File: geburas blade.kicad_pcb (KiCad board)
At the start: 2 copper layers, 71.8 x 71.8 mm, 17 parts, among them M1 Motor_DC, Q1 2N3904, SW2 SW_Push, U2 ICM7555xP

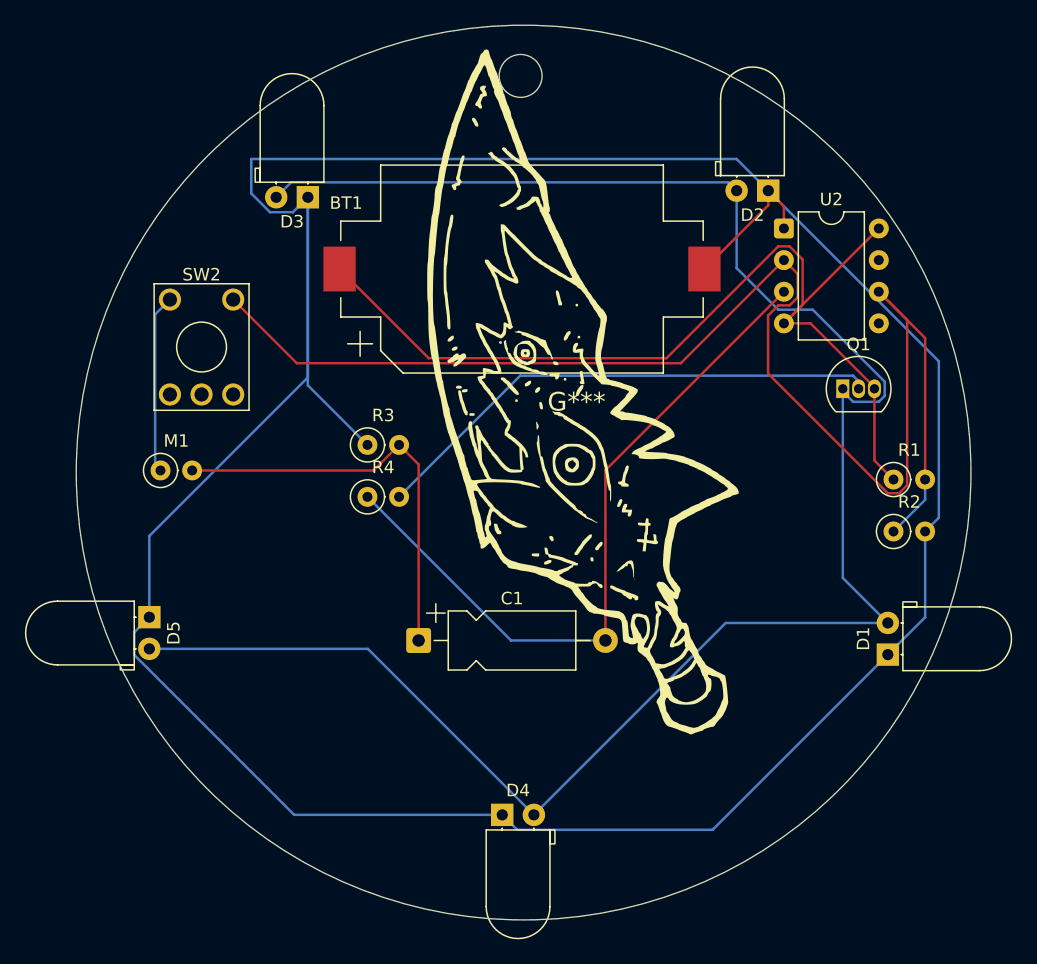
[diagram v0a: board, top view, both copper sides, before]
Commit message: Add files via upload
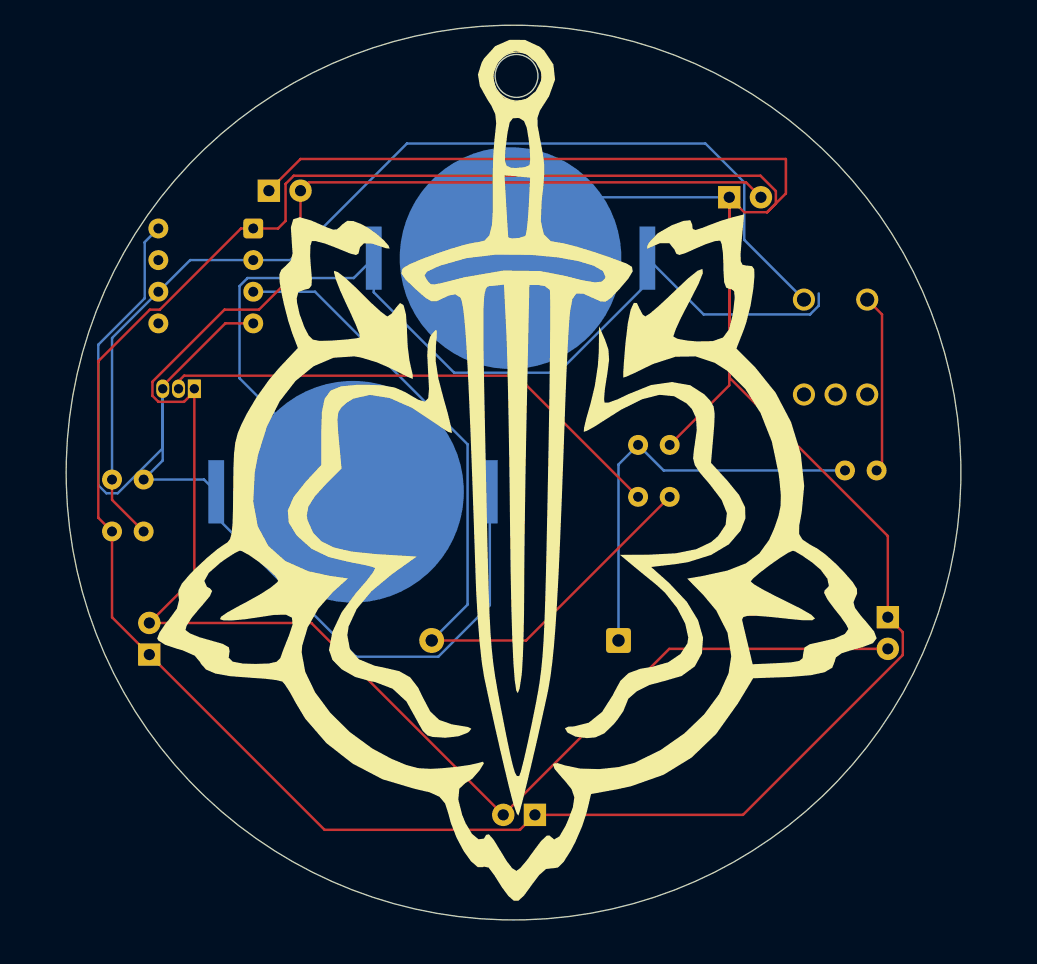
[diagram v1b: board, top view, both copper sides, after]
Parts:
- added BT2: Battery_Cell, Battery:BatteryHolder_Keystone_3034_1x20mm, B.Cu at (128.5, 76.5)
- BT1: footprint Battery:BatteryHolder_Keystone_1060_1x2032 -> Battery:BatteryHolder_Keystone_3034_1x20mm; moved to B.Cu
- C1, D1, D2, D3, D4, D5, G***, M1, Q1, R1, R2, R3, R4, SW2, U2: moved to B.Cu
- G***: moved to F.Cu
- moved R1 60.2 mm to (111.7, 75.5), turned to 180 degrees
- moved R2 60.2 mm to (111.7, 79.7), turned to 180 degrees
- moved D1 59.3 mm to (112.2, 89.5)
- moved D5 59.3 mm to (171.5, 86.5)
- moved M1 57.5 mm to (170.6, 74.8), turned to 180 degrees
- moved SW2 56.0 mm to (169.8, 61.0), turned to 180 degrees
- moved Q1 52.1 mm to (115.8, 68.2), turned to 180 degrees
- moved U2 42.6 mm to (120.5, 55.3), turned to 180 degrees
- moved D2 40.1 mm to (121.8, 52.3), turned to 0 degrees
- moved D3 33.8 mm to (158.8, 52.8), turned to 0 degrees
- moved R3 24.3 mm to (154.0, 72.7), turned to 180 degrees
- moved R4 24.3 mm to (154.0, 76.9), turned to 180 degrees
- moved C1 16.1 mm to (149.9, 88.4), turned to 180 degrees
- moved G*** 9.31 mm to (137.2, 69.3), turned to 180 degrees
- moved D4 2.62 mm to (143.1, 102.4), turned to 180 degrees
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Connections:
- Q1 pad 3: Net-(BT1-+) -> Net-(BT2-+)
- R1 pad 1: Net-(BT1-+) -> Net-(BT2-+)
- U2 pad 4: Net-(BT1-+) -> Net-(BT2-+)
- U2 pad 8: Net-(BT1-+) -> Net-(BT2-+)
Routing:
- net Net-(BT2-+): track 0.00 -> 97.6 mm
- net Net-(BT1--): track 244.1 -> 297.2 mm
- net Net-(U2-THRES): track 114.6 -> 86.5 mm
- net Net-(U2-OUT): track 57.8 -> 63.1 mm
- net Net-(BT1-+): track 78.3 -> 81.3 mm
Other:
- outline, holes or cut-outs redrawn
